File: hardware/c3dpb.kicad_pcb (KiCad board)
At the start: 4 copper layers, 100 x 75 mm, 567 parts, among them IC1 TMC5161, IC2 TMC5161, IC3 TMC5161, IC4 TMC5161, IC5 TMC5161, J1 Conn_01x01, J10 Conn_01x01, J100 Conn_01x01, J101 Conn_01x01, J102 Conn_01x01, J104 Conn_01x01, J11 Conn_01x01, J12 Conn_01x01, J13 Conn_01x01, J14 Conn_01x01, J15 Conn_01x01, J16 Conn_01x01, J17 Conn_01x01, J18 Conn_01x01, J19 Conn_01x01, J2 Conn_01x01, J20 Conn_01x01, J21 Conn_01x01, J22 Conn_01x01, J23 Conn_01x01, J24 Conn_01x01, J25 Conn_01x01, J26 Conn_01x01, J27 Conn_01x01, J28 Conn_01x01, J29 Conn_01x01, J3 Conn_01x01, J30 Conn_01x01, J31 Conn_01x01, J32 Conn_01x01, J33 Conn_01x01, J34 Conn_01x01, J35 Conn_01x01, J36 Conn_01x01, J37 Conn_01x01, J38 Conn_01x01, J39 Screw_Terminal_01x02, J4 Conn_01x01, J44 Conn_01x01, J45 Conn_01x01, J46 Conn_01x03, J47 Conn_01x03, J48 Conn_01x01, J49 Conn_01x01, J5 Conn_01x01, J50 Conn_01x01, J51 Conn_01x01, J52 Conn_01x01, J53 Conn_01x01, J54 Conn_01x01, J55 Conn_01x01, J56 Conn_01x01, J57 Conn_01x01, J58 Conn_01x01, J59 Conn_01x01, J6 Conn_01x01, J60 USB_C_Receptacle, J61 Micro_SD_Card_Det, J62 Conn_01x02, J63 Conn_01x02, J66 Conn_01x03, J67 Conn_01x03, J68 Conn_01x01, J69 Conn_01x01, J7 Conn_01x01, J70 Conn_01x01, J71 Conn_01x02, J72 Conn_01x02, J73 Conn_01x02, J74 Conn_01x02, J75 Conn_01x01, J76 Conn_01x01, J77 Conn_01x01, J78 Conn_01x01, J79 Conn_01x03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

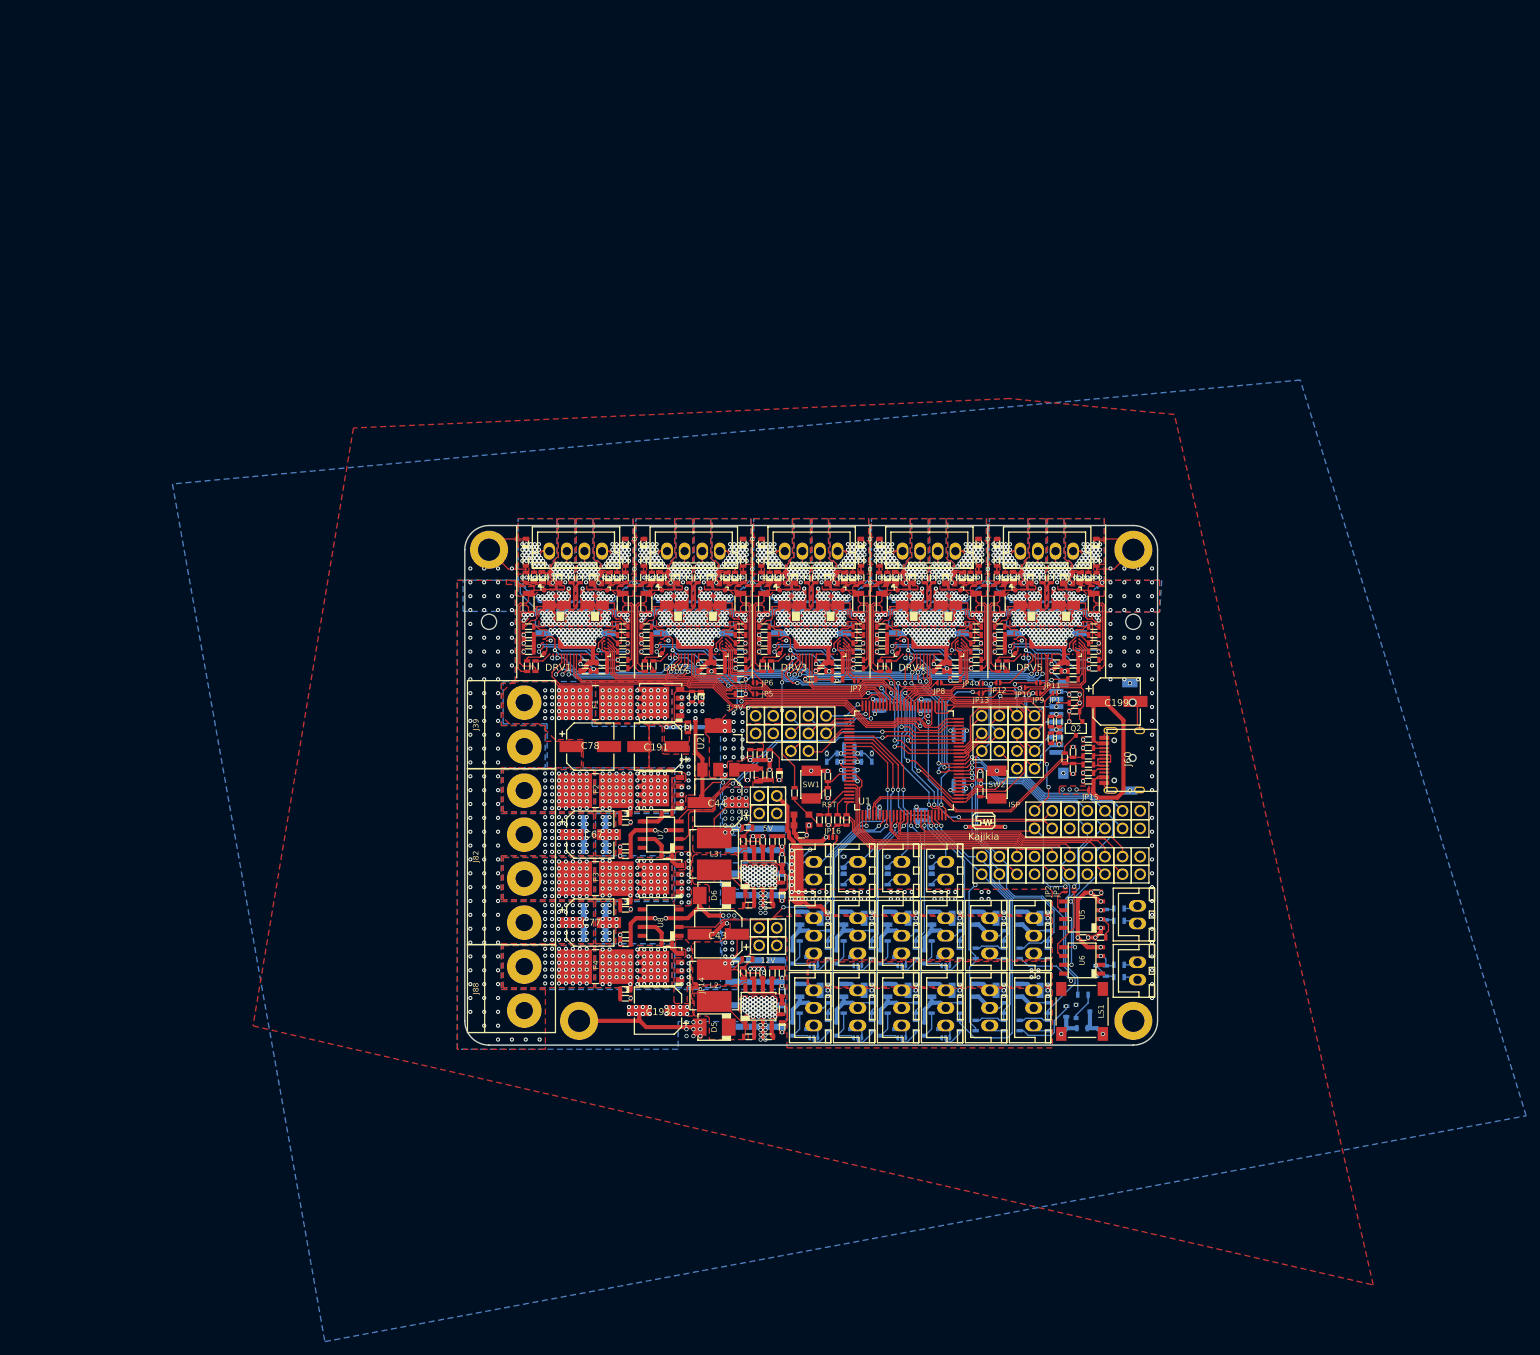
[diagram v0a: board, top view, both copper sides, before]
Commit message: layout
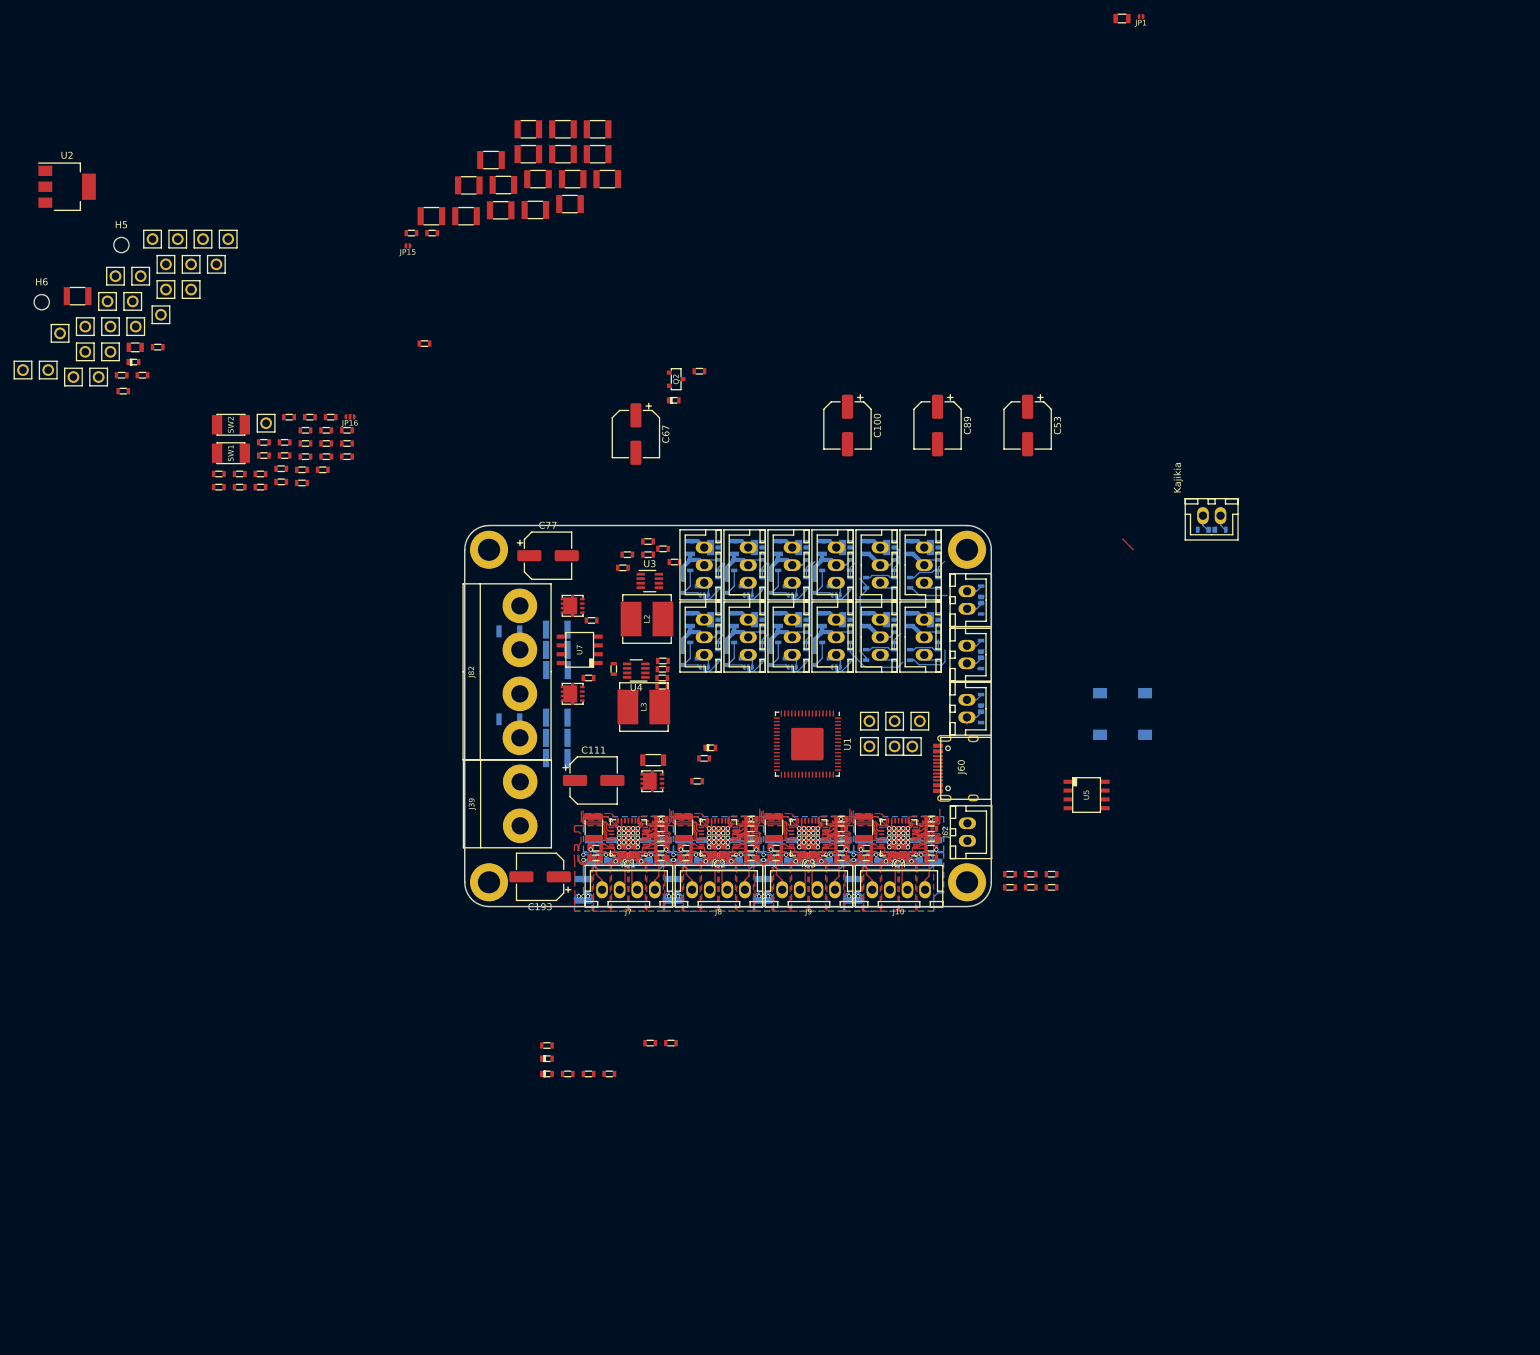
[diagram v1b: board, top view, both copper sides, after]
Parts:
- removed C130, C145, C148, C150, C151, C166, C169, C171, C172: 100n, _Generic:0603_CAP
- removed C131, C132, C134, C135, C142, C143, C147, C152, C153, C155, C156, C163, C164, C168, C173, C174, C176, C177, C184, C185: 470n, _Generic:0603_CAP
- removed C133, C136, C137, C154, C157, C158, C175, C178, C179, C186, C187, C188, C189, C190, C194, C195, C196, C197: 4.7u, _Generic:1210_CAP
- removed C138, C139, C140, C141, C159, C160, C161, C162, C180, C181, C182, C183: 470p, _Generic:0603_CAP
- removed C144, C146, C165, C167: 10u, _Generic:0603_CAP
- removed C149, C170: 22n, _Generic:0603_CAP
- removed C191, C199: 220u, Capacitor_SMD:CP_Elec_6.3x7.7
- removed D25: LED, _Generic:0603_LED
- removed D26, D27, D28, D29, D30, D31, D32, D33, D34, D35, D36, D37, D38, D39, D40, D41, D42, D43, D44, D45, D46, D47, D48, D49, D50, D51, D52, D53, D54, D55, D56, D57, D58, D59, D60, D61, D62, D63, D64, D65, D66: MSK4010, _Generic:SOD-523_DIODE
- removed D3: 3.6v, _Generic:SOD-523_DIODE
- removed D5, D6: SK54, _Generic:SMB_DIODE
- removed F4: Fuse, _Generic:SMD_Fuseholder
- removed IC5: TMC5161, footprints:QFN42L
- removed J104, J11, J12, J13, J14, J15, J16, J17, J18, J19, J20, J21, J22, J23, J25, J26, J27, J28, J29, J30, J31, J32, J33, J34, J35, J36, J37, J38, J52, J75, J76, J77, J78: Conn_01x01, _Generic:PinHeader_2.54mm_1P
- removed J61: Micro_SD_Card_Det, _Generic:HYC77-TF09-200
- removed J63: Conn_01x02, _Generic:JST_XH_2P
- removed J88: Screw_Terminal_01x02, _Generic:KF635-2P
- removed J89, J90, J91, J92, J93: Conn_01x04, _Generic:JST_XH_4P
- removed JP10, JP11, JP12, JP13, JP14, JP2, JP3, JP38, JP39, JP4, JP40, JP41, JP42, JP5, JP6, JP7, JP8, JP9: SolderJumper_2_Open, _Generic:Solder Jumper 2P
- removed L6, L7: 470, _Generic:0603_IND
- removed Q11: AON6144, _Generic:DFN5x6-8
- removed Q14: AO3400, _Generic:SOT-23
- removed R100, R109, R118, R82, R91: 2.2R, _Generic:0603_RES
- removed R101, R110, R119, R76, R77, R80, R83, R92: 1k, _Generic:0603_RES
- removed R102, R103, R104, R105, R111, R112, R113, R114, R120, R121, R122, R123, R84, R85, R86, R87, R93, R94, R95, R96: 47R, _Generic:0603_RES
- removed R106, R107, R115, R116, R124, R125, R88, R89, R97, R98: 100m, _Generic:1206_RES
- removed R108, R117, R34, R78, R81, R90, R99: 0R, _Generic:0603_RES
- removed R30, R31, R79: 10k, _Generic:0603_RES
- removed R75: 10R, _Generic:0603_RES
- removed U6: MAX6675, _Generic:SO-8
- removed U8: IR4427S, _Generic:SO-8
- removed X1: 12MHz, Oscillator:Oscillator_SMD_EuroQuartz_XO32-4Pin_3.2x2.5mm
- added FB1: Ferrite_Bead_Small, _Generic:0805_IND, F.Cu at (194.9, -23.2)
- C10, C11, C12, C13, C14, C15, C16, C17, C19, C2, C23, C24, C25, C26, C27, C31, C4, C48, C6, C7, C8, C9, L4, L5, R4, R5, R6, R7: moved to F.Cu
- C100, C111, C89: value 470n -> 100u; footprint _Generic:0603_CAP -> Capacitor_SMD:CP_Elec_6.3x7.7
- C101, C114, C90, C92: value 470n -> 470p; moved to B.Cu
- C102, C104: value 10u -> 470p
- C103: value 100n -> 470p; moved to B.Cu
- C105: value 470n -> 100n
- C106, C127, C129, C47, C52, C88: value 100n -> 4.7u; footprint _Generic:0603_CAP -> _Generic:1210_CAP; moved to B.Cu
- C107: value 22n -> 2.2u
- C109, C87: value 100n -> 22n
- C110, C121, C84: value 470n -> 4.7u; footprint _Generic:0603_CAP -> _Generic:1210_CAP; moved to B.Cu
- C112: value 4.7u -> 470p; footprint _Generic:1210_CAP -> _Generic:0603_CAP
- C113, C93: value 470n -> 470p
- C115, C91: value 4.7u -> 470p; footprint _Generic:1210_CAP -> _Generic:0603_CAP; moved to F.Cu
- C116, C94: value 4.7u -> 100n; footprint _Generic:1210_CAP -> _Generic:0603_CAP; moved to F.Cu
- C117, C118, C119, C97: value 470p -> 100n
- C120: value 470p -> 4.7u; footprint _Generic:0603_CAP -> _Generic:1210_CAP
- C122, C126: value 470n -> 4.7u; footprint _Generic:0603_CAP -> _Generic:1210_CAP
- C123, C125: value 10u -> 4.7u; footprint _Generic:0603_CAP -> _Generic:1210_CAP; moved to B.Cu
- C124, C5: value 100n -> 4.7u; footprint _Generic:0603_CAP -> _Generic:1210_CAP
- C128: value 22n -> 4.7u; footprint _Generic:0603_CAP -> _Generic:1210_CAP; moved to B.Cu
- C28: value 4.7u -> 10n; footprint _Generic:1210_CAP -> _Generic:0603_CAP; moved to F.Cu
- C29: value 100n -> 47p
- C3: value 220p -> 4.7u; footprint _Generic:0603_CAP -> _Generic:1210_CAP
- C30, C38: value 100n -> 22u; footprint _Generic:0603_CAP -> _Generic:1210_CAP
- C32, C41, C42: value 4.7u -> 22u; moved to F.Cu
- C33, C34: value 22n -> 22u; footprint _Generic:0603_CAP -> _Generic:1210_CAP
- C35, C36: value 12p -> 22u; footprint _Generic:0603_CAP -> _Generic:1210_CAP
- C37: value 100n -> 10n
- C39: value DNP -> 47p
- C40: value DNP -> 22u; footprint _Generic:0603_CAP -> _Generic:1210_CAP
- C43, C44: value 220u -> 22u; footprint Capacitor_SMD:CP_Elec_6.3x7.7 -> _Generic:1210_CAP
- C46, C83: value 10u -> 100n
- C49: value 10u -> 2.2u
- C50: value 12p -> 100n
- C51: value 12p -> 22n
- C53: value 22n -> 100u; footprint _Generic:0603_CAP -> Capacitor_SMD:CP_Elec_6.3x7.7; moved to F.Cu
- C78: value 220u -> 470p; footprint Capacitor_SMD:CP_Elec_6.3x7.7 -> _Generic:0603_CAP; moved to B.Cu
- C80: value 100p -> 470p
- C81: value 10u -> 470p; moved to B.Cu
- C82: value 100n -> 470p
- C85: value 100n -> 2.2u
- C86: value 22n -> 100n
- C96: value 470p -> 2.2u
- C98: value 470p -> 22n
- C99: value 470p -> 4.7u; footprint _Generic:0603_CAP -> _Generic:1210_CAP; moved to B.Cu
- D2: value 3.6v -> MSK4010
- F1: footprint _Generic:SMD_Fuseholder -> _Generic:1206_RES
- F2, F3: footprint _Generic:SMD_Fuseholder -> _Generic:1206_RES; moved to B.Cu
- IC1, IC2, IC3, IC4: value TMC5161 -> TMC2209; footprint footprints:QFN42L -> Package_DFN_QFN:QFN-28-1EP_5x5mm_P0.5mm_EP3.35x3.35mm
- J10, J7, J8, J9: value Conn_01x01 -> Conn_01x04; footprint _Generic:PinHeader_2.54mm_1P -> _Generic:JST_XH_4P
- LS1: moved to B.Cu
- Q1, Q6, Q7: value AON6144 -> AON7418; footprint _Generic:DFN5x6-8 -> _Generic:DFN3x3A_8L_EP1_P
- Q2: value AO3401 -> AO3400
- R10: value 47k -> 1k
- R11: value 47k -> 100k
- R12, R17: value 140k -> 100k
- R13: value 140k -> 13.3k
- R16: value 100k -> 1k
- R18: value 10k -> 4.7k
- R19: value 52.3k -> 120m; footprint _Generic:0603_RES -> _Generic:1206_RES; moved to B.Cu
- R20, R27, R29: value 10k -> 120m; footprint _Generic:0603_RES -> _Generic:1206_RES; moved to B.Cu
- R24, R25: value 47R -> 120m; footprint _Generic:0603_RES -> _Generic:1206_RES; moved to B.Cu
- R26: value 1.5k -> 120m; footprint _Generic:0603_RES -> _Generic:1206_RES; moved to B.Cu
- R28: value 47k -> 120m; footprint _Generic:0603_RES -> _Generic:1206_RES; moved to B.Cu
- R8: value 10k -> 100k
- R9: value 100k -> 1meg
- U1: value LPC1769FBD100 -> ATSAMD51J19A-M; footprint Package_QFP:LQFP-100_14x14mm_P0.5mm -> Package_DFN_QFN:QFN-64-1EP_9x9mm_P0.5mm_EP4.7x4.7mm
- U3, U4: value AOZ1284 -> SY8303; footprint _Generic:SO-8-EP1 -> Package_TO_SOT_SMD:TSOT-23-8
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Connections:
- net Net-(IC2-Pad9) renamed /Driver 3/AD0
- net Net-(IC4-Pad9) renamed /Driver 1/AD0
- C101 pad 1: +24V -> Net-(C101-Pad1)
- C103 pad 1: Net-(C102-Pad1) -> Net-(C103-Pad1)
- C104 pad 1: /Stepper Driver/Driver2/5V_out -> Net-(C104-Pad1)
- C105 pad 1: /Stepper Driver/Driver2/VCC -> GND
- C105 pad 2: GND -> +24V
- C106 pad 1: +3V3 -> +24V
- C107 pad 2: Net-(C107-Pad2) -> GND
- C109 pad 1: GND -> Net-(C109-Pad1)
- C109 pad 2: +24V -> Net-(C109-Pad2)
- C110 pad 1: /Stepper Driver/Driver2/OA2 -> +24V
- C110 pad 2: Net-(C110-Pad2) -> GND
- C111 pad 1: /Stepper Driver/Driver2/OB2 -> +24V
- C111 pad 2: Net-(C111-Pad2) -> GND
- C112 pad 1: +24V -> Net-(C112-Pad1)
- C113 pad 1: /Stepper Driver/Driver2/OA1 -> Net-(C113-Pad1)
- C113 pad 2: Net-(C113-Pad2) -> GND
- C114 pad 1: /Stepper Driver/Driver2/OB1 -> Net-(C114-Pad1)
- C114 pad 2: Net-(C114-Pad2) -> GND
- C115 pad 1: +24V -> Net-(C115-Pad1)
- C116 pad 1: +24V -> GND
- C116 pad 2: GND -> +24V
- C117 pad 1: /Stepper Driver/Driver2/OA2 -> GND
- C117 pad 2: GND -> +24V
- C118 pad 1: /Stepper Driver/Driver2/OB2 -> GND
- C118 pad 2: GND -> +24V
- C119 pad 1: /Stepper Driver/Driver2/OA1 -> GND
- C119 pad 2: GND -> +24V
- C120 pad 1: /Stepper Driver/Driver2/OB1 -> +24V
- C123 pad 1: Net-(C123-Pad1) -> +24V
- C124 pad 1: Net-(C123-Pad1) -> +24V
- C125 pad 1: /Stepper Driver/Driver3/5V_out -> +24V
- C126 pad 1: /Stepper Driver/Driver3/VCC -> +24V
- C127 pad 1: +3V3 -> +24V
- C128 pad 2: Net-(C128-Pad2) -> DCIN-
- C129 pad 2: +24V -> DCIN-
- C192 pad 1: +24V -> Net-(C129-Pad1)
- C198 pad 1: VBUS -> Net-(C198-Pad1)
- C28 pad 1: +24V -> Net-(C28-Pad1)
- C28 pad 2: GND -> Net-(C28-Pad2)
- C29 pad 1: Net-(C29-Pad1) -> +5V
- C29 pad 2: GND -> Net-(C29-Pad2)
- C3 pad 1: /LPC_CLK -> +24V
- C30 pad 1: Net-(C30-Pad1) -> +12V
- C30 pad 2: GND -> Net-(C30-Pad2)
- C32 pad 1: +24V -> +12V
- C33 pad 1: Net-(C33-Pad1) -> +5V
- C33 pad 2: GND -> Net-(C33-Pad2)
- C34 pad 1: Net-(C34-Pad1) -> +5V
- C35 pad 1: Net-(C35-Pad1) -> +12V
- C35 pad 2: Net-(C35-Pad2) -> Net-(C30-Pad2)
- C36 pad 1: Net-(C36-Pad1) -> +12V
- C36 pad 2: Net-(C36-Pad2) -> GND
- C38 pad 1: Net-(C38-Pad1) -> +5V
- C38 pad 2: Net-(C38-Pad2) -> Net-(C33-Pad2)
- C40 pad 2: Net-(C40-Pad2) -> GND
- C41 pad 2: GND -> Net-(C30-Pad2)
- C42 pad 1: +5V -> +12V
- C43 pad 1: +12V -> +5V
- C43 pad 2: GND -> Net-(C33-Pad2)
- C46 pad 1: VBUS -> GND
- C46 pad 2: GND -> +24V
- C47 pad 1: +3V3 -> +24V
- C49 pad 1: +3V3 -> Net-(C49-Pad1)
- C5 pad 1: +3V3 -> +24V
- C50 pad 1: /USB_D+ -> Net-(C50-Pad1)
- C50 pad 2: GND -> +24V
- C51 pad 1: /USB_D- -> Net-(C51-Pad1)
- C51 pad 2: GND -> Net-(C51-Pad2)
- C52 pad 1: +3V3 -> +24V
- C53 pad 1: Net-(C53-Pad1) -> +24V
- C53 pad 2: Net-(C53-Pad2) -> GND
- C68 pad 1: +24V -> Net-(C129-Pad1)
- C69 pad 1: +24V -> Net-(C128-Pad1)
- C78 pad 1: +24V -> Net-(C78-Pad1)
- C78 pad 2: DCIN- -> GND
- C79 pad 1: +24V -> Net-(C128-Pad1)
- C80 pad 1: /LPC_CLK -> Net-(C80-Pad1)
- C80 pad 2: Net-(C80-Pad2) -> GND
- C82 pad 1: Net-(C81-Pad1) -> Net-(C82-Pad1)
- C83 pad 1: /Stepper Driver/Driver1/5V_out -> GND
- C83 pad 2: GND -> +24V
- C84 pad 1: /Stepper Driver/Driver1/VCC -> +24V
- C85 pad 1: +3V3 -> Net-(C85-Pad1)
- C86 pad 2: Net-(C86-Pad2) -> +24V
- C87 pad 2: +24V -> Net-(C87-Pad2)
- C88 pad 1: GND -> +24V
- C88 pad 2: +24V -> GND
- C89 pad 1: /Stepper Driver/Driver1/OA2 -> +24V
- C89 pad 2: Net-(C89-Pad2) -> GND
- C90 pad 1: /Stepper Driver/Driver1/OB2 -> Net-(C90-Pad1)
- C90 pad 2: Net-(C90-Pad2) -> GND
- C91 pad 1: +24V -> Net-(C91-Pad1)
- C92 pad 1: /Stepper Driver/Driver1/OA1 -> Net-(C92-Pad1)
- C92 pad 2: Net-(C92-Pad2) -> GND
- C93 pad 1: /Stepper Driver/Driver1/OB1 -> Net-(C93-Pad1)
- C93 pad 2: Net-(C93-Pad2) -> GND
- C94 pad 1: +24V -> GND
- C94 pad 2: GND -> +24V
- C96 pad 1: /Stepper Driver/Driver1/OA2 -> Net-(C96-Pad1)
- C97 pad 1: /Stepper Driver/Driver1/OB2 -> Net-(C97-Pad1)
- C97 pad 2: GND -> +24V
- C98 pad 1: /Stepper Driver/Driver1/OA1 -> Net-(C98-Pad1)
- C98 pad 2: GND -> Net-(C98-Pad2)
- C99 pad 1: /Stepper Driver/Driver1/OB1 -> +24V
- D2 pad 1: Net-(C29-Pad1) -> +3V3
- D2 pad 2: GND -> Net-(D2-Pad2)
- F2 pad 1: Net-(F2-Pad1) -> Net-(C128-Pad1)
- F2 pad 2: Net-(D18-Pad1) -> +24V
- F3 pad 1: Net-(F3-Pad1) -> Net-(C129-Pad1)
- F3 pad 2: Net-(D19-Pad1) -> +24V
- IC1 pad 1: Net-(C93-Pad2) -> Net-(C82-Pad1)
- IC1 pad 10: Net-(IC1-Pad10) -> /Driver 2/AD1
- IC1 pad 11: /Stepper Driver/Driver1/SRBH -> /DRV2_DIAG
- IC1 pad 14: /DRV_CLK -> /DRV_UART
- IC1 pad 15: /DRV1_CS -> Net-(IC1-Pad15)
- IC1 pad 16: /DRV_SCK -> /DRV2_STEP
- IC1 pad 17: /DRV_MOSI -> Net-(IC1-Pad17)
- IC1 pad 18: /DRV_MISO -> GND
- IC1 pad 19: /DRV1_STEP -> /DRV2_DIR
- IC1 pad 2: Net-(C81-Pad1) -> /DRV2_EN
- IC1 pad 20: /DRV1_DIR -> Net-(IC1-Pad20)
- IC1 pad 21: +3V3 -> Net-(C80-Pad1)
- IC1 pad 22: +3V3 -> +24V
- IC1 pad 23: +3V3 -> Net-(IC1-Pad23)
- IC1 pad 24: GND -> Net-(C78-Pad1)
- IC1 pad 25: GND -> Net-(IC1-Pad25)
- IC1 pad 26: GND -> Net-(C81-Pad1)
- IC1 pad 28: Net-(IC1-Pad28) -> +24V
- IC1 pad 29: /Stepper Driver/DRV1_DIAG1 -> GND
- IC1 pad 3: Net-(IC1-Pad3) -> GND
- IC1 pad 4: Net-(C81-Pad1) -> Net-(C51-Pad2)
- IC1 pad 5: /Stepper Driver/Driver1/5V_out -> Net-(C51-Pad1)
- IC1 pad 6: /Stepper Driver/Driver1/5V_out -> Net-(C50-Pad1)
- IC1 pad 7: GND -> Net-(IC1-Pad7)
- IC1 pad 8: Net-(IC1-Pad8) -> Net-(C49-Pad1)
- IC1 pad 9: Net-(IC1-Pad9) -> +3V3
- IC2 pad 1: Net-(C114-Pad2) -> Net-(C93-Pad1)
- IC2 pad 10: Net-(IC2-Pad10) -> +3V3
- IC2 pad 11: /Stepper Driver/Driver2/SRBH -> /DRV3_DIAG
- IC2 pad 14: /DRV_CLK -> /DRV_UART
- IC2 pad 15: /DRV2_CS -> Net-(IC2-Pad15)
- IC2 pad 16: /DRV_SCK -> /DRV3_STEP
- IC2 pad 17: /DRV_MOSI -> Net-(IC2-Pad17)
- IC2 pad 18: /DRV_MISO -> GND
- IC2 pad 19: /DRV2_STEP -> /DRV3_DIR
- IC2 pad 2: Net-(C102-Pad1) -> /DRV3_EN
- IC2 pad 20: /DRV2_DIR -> Net-(IC2-Pad20)
- IC2 pad 21: +3V3 -> Net-(C91-Pad1)
- IC2 pad 22: +3V3 -> +24V
- IC2 pad 23: +3V3 -> Net-(IC2-Pad23)
- IC2 pad 24: GND -> Net-(C90-Pad1)
- IC2 pad 25: GND -> Net-(IC2-Pad25)
- IC2 pad 26: GND -> Net-(C92-Pad1)
- IC2 pad 28: Net-(IC2-Pad28) -> +24V
- IC2 pad 29: /Stepper Driver/DRV2_DIAG1 -> GND
- IC2 pad 3: Net-(IC2-Pad3) -> GND
- IC2 pad 4: Net-(C102-Pad1) -> Net-(C87-Pad2)
- IC2 pad 5: /Stepper Driver/Driver2/5V_out -> Net-(C87-Pad1)
- IC2 pad 6: /Stepper Driver/Driver2/5V_out -> Net-(C86-Pad1)
- IC2 pad 7: GND -> Net-(IC2-Pad7)
- IC2 pad 8: Net-(IC2-Pad8) -> Net-(C85-Pad1)
- IC3 pad 1: Net-(C135-Pad2) -> Net-(C104-Pad1)
- IC3 pad 10: Net-(IC3-Pad10) -> +3V3
- IC3 pad 11: /Stepper Driver/Driver3/SRBH -> /DRV4_DIAG
- IC3 pad 14: /DRV_CLK -> /DRV_UART
- IC3 pad 15: /DRV3_CS -> Net-(IC3-Pad15)
- IC3 pad 16: /DRV_SCK -> /DRV4_STEP
- IC3 pad 17: /DRV_MOSI -> Net-(IC3-Pad17)
- IC3 pad 18: /DRV_MISO -> GND
- IC3 pad 19: /DRV3_STEP -> /DRV4_DIR
- IC3 pad 2: Net-(C123-Pad1) -> /DRV4_EN
- IC3 pad 20: /DRV3_DIR -> Net-(IC3-Pad20)
- IC3 pad 21: +3V3 -> Net-(C102-Pad1)
- IC3 pad 22: +3V3 -> +24V
- IC3 pad 23: +3V3 -> Net-(IC3-Pad23)
- IC3 pad 24: GND -> Net-(C101-Pad1)
- IC3 pad 25: GND -> Net-(IC3-Pad25)
- IC3 pad 26: GND -> Net-(C103-Pad1)
- IC3 pad 28: Net-(IC3-Pad28) -> +24V
- IC3 pad 29: /Stepper Driver/DRV3_DIAG1 -> GND
- IC3 pad 3: Net-(IC3-Pad3) -> GND
- IC3 pad 4: Net-(C123-Pad1) -> Net-(C98-Pad2)
- IC3 pad 5: /Stepper Driver/Driver3/5V_out -> Net-(C98-Pad1)
- IC3 pad 6: /Stepper Driver/Driver3/5V_out -> Net-(C97-Pad1)
- IC3 pad 7: GND -> Net-(IC3-Pad7)
- IC3 pad 8: Net-(IC3-Pad8) -> Net-(C96-Pad1)
- IC3 pad 9: Net-(IC3-Pad9) -> +3V3
- IC4 pad 1: Net-(C156-Pad2) -> Net-(C115-Pad1)
- IC4 pad 10: Net-(IC4-Pad10) -> /Driver 1/AD1
- IC4 pad 11: /Stepper Driver/Driver4/SRBH -> /DRV1_DIAG
- IC4 pad 14: /DRV_CLK -> /DRV_UART
- IC4 pad 15: /DRV4_CS -> Net-(IC4-Pad15)
- IC4 pad 16: /DRV_SCK -> /DRV1_STEP
- IC4 pad 17: /DRV_MOSI -> Net-(IC4-Pad17)
- IC4 pad 18: /DRV_MISO -> GND
- IC4 pad 19: /DRV4_STEP -> /DRV1_DIR
- IC4 pad 2: Net-(C144-Pad1) -> /DRV1_EN
- IC4 pad 20: /DRV4_DIR -> Net-(IC4-Pad20)
- IC4 pad 21: +3V3 -> Net-(C113-Pad1)
- IC4 pad 22: +3V3 -> +24V
- IC4 pad 23: +3V3 -> Net-(IC4-Pad23)
- IC4 pad 24: GND -> Net-(C112-Pad1)
- IC4 pad 25: GND -> Net-(IC4-Pad25)
- IC4 pad 26: GND -> Net-(C114-Pad1)
- IC4 pad 28: Net-(IC4-Pad28) -> +24V
- IC4 pad 29: /Stepper Driver/DRV4_DIAG1 -> GND
- IC4 pad 3: Net-(IC4-Pad3) -> GND
- IC4 pad 4: Net-(C144-Pad1) -> Net-(C109-Pad2)
- IC4 pad 5: /Stepper Driver/Driver4/5V_out -> Net-(C109-Pad1)
- IC4 pad 6: /Stepper Driver/Driver4/5V_out -> Net-(C108-Pad1)
- IC4 pad 7: GND -> Net-(IC4-Pad7)
- IC4 pad 8: Net-(IC4-Pad8) -> Net-(C107-Pad1)
- J1 pad 1: /P0.0_END -> /SWCLK
- J10 pad 1: /DRV5_CS -> Net-(C115-Pad1)
- J2 pad 1: /P0.1_END -> /BUZZER
- J3 pad 1: /P0.2 -> Net-(J3-Pad1)
- J4 pad 1: /P0.3 -> Net-(J4-Pad1)
- J5 pad 1: /SD_CS -> Net-(J5-Pad1)
- J6 pad 1: /SD_SCK -> Net-(J6-Pad1)
- J60 pad A4: VBUS -> Net-(C198-Pad1)
- J60 pad A6: Net-(J60-PadA6) -> /USB_D+
- J60 pad A7: Net-(J60-PadA7) -> /USB_D-
- J60 pad A9: VBUS -> Net-(C198-Pad1)
- J60 pad B4: VBUS -> Net-(C198-Pad1)
- J60 pad B6: Net-(J60-PadA6) -> /USB_D+
- J60 pad B7: Net-(J60-PadA7) -> /USB_D-
- J60 pad B9: VBUS -> Net-(C198-Pad1)
- J60 pad S1: GND -> Net-(FB1-Pad2)
- J7 pad 1: /SD_MISO -> Net-(C82-Pad1)
- J8 pad 1: /SD_MOSI -> Net-(C93-Pad1)
- J82 pad 1: Net-(F2-Pad1) -> Net-(D18-Pad1)
- J82 pad 2: +24V -> Net-(C128-Pad1)
- J82 pad 3: Net-(F3-Pad1) -> Net-(D19-Pad1)
- J82 pad 4: +24V -> Net-(C129-Pad1)
- J9 pad 1: /DRV_SCK -> Net-(C104-Pad1)
- JP1 pad 1: /Interfaces/SD_DETECT -> /BUZZER
- JP1 pad 2: /P4.29 -> Net-(JP1-Pad2)
- JP15 pad 1: VBUS -> Net-(C198-Pad1)
- L3 pad 1: Net-(C38-Pad2) -> Net-(C28-Pad2)
- LS1 pad 1: Net-(D26-Pad1) -> +3V3
- LS1 pad 2: Net-(D26-Pad2) -> Net-(D2-Pad2)
- Q2 pad 1: /USB_CON -> Net-(Q2-Pad1)
- Q2 pad 2: +3V3 -> GND
- Q2 pad 3: Net-(Q2-Pad3) -> Net-(D2-Pad2)
- R10 pad 1: Net-(R10-Pad1) -> +3V3
- R10 pad 2: GND -> /SWCLK
- R12 pad 1: +24V -> +5V
- R12 pad 2: Net-(C29-Pad1) -> Net-(C29-Pad2)
- R13 pad 1: +24V -> Net-(C29-Pad2)
- R13 pad 2: Net-(C30-Pad1) -> GND
- R15 pad 1: Net-(C35-Pad2) -> Net-(R15-Pad1)
- R16 pad 1: Net-(C36-Pad2) -> Net-(Q2-Pad1)
- R16 pad 2: GND -> Net-(JP1-Pad2)
- R19 pad 1: +5V -> Net-(IC1-Pad27)
- R19 pad 2: Net-(C40-Pad2) -> GND
- R20 pad 1: Net-(C40-Pad2) -> Net-(IC1-Pad23)
- R24 pad 1: /USB_D- -> Net-(IC2-Pad27)
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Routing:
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- added copper zone on B.Cu, net Net-(C101-Pad1)
- added copper zone on F.Cu, net Net-(C101-Pad1)
- added copper zone on F.Cu, net Net-(C102-Pad1)
- added copper zone on B.Cu, net Net-(C103-Pad1)
- added copper zone on F.Cu, net Net-(C103-Pad1)
- added copper zone on F.Cu, net Net-(C104-Pad1)
- added copper zone on F.Cu, net Net-(C107-Pad1)
- added copper zone on F.Cu, net Net-(C108-Pad1)
- added copper zone on F.Cu, net Net-(C109-Pad1)
- added copper zone on F.Cu, net Net-(C109-Pad2)
- added copper zone on B.Cu, net Net-(C112-Pad1)
- added copper zone on F.Cu, net Net-(C112-Pad1)
- added copper zone on F.Cu, net Net-(C113-Pad1)
- added copper zone on B.Cu, net Net-(C114-Pad1)
- added copper zone on F.Cu, net Net-(C114-Pad1)
- added copper zone on F.Cu, net Net-(C115-Pad1)
- added copper zone on F.Cu, net Net-(C49-Pad1)
- added copper zone on F.Cu, net Net-(C50-Pad1)
- added copper zone on F.Cu, net Net-(C51-Pad1)
- added copper zone on F.Cu, net Net-(C51-Pad2)
- added copper zone on B.Cu, net Net-(C78-Pad1)
- added copper zone on F.Cu, net Net-(C78-Pad1)
- added copper zone on F.Cu, net Net-(C80-Pad1)
- added copper zone on B.Cu, net Net-(C81-Pad1)
- added copper zone on F.Cu, net Net-(C81-Pad1)
- added copper zone on F.Cu, net Net-(C82-Pad1)
- added copper zone on F.Cu, net Net-(C85-Pad1)
- added copper zone on F.Cu, net Net-(C86-Pad1)
- added copper zone on F.Cu, net Net-(C87-Pad1)
- added copper zone on F.Cu, net Net-(C87-Pad2)
- added copper zone on B.Cu, net Net-(C90-Pad1)
- added copper zone on F.Cu, net Net-(C90-Pad1)
- added copper zone on F.Cu, net Net-(C91-Pad1)
- added copper zone on B.Cu, net Net-(C92-Pad1)
- added copper zone on F.Cu, net Net-(C92-Pad1)
- added copper zone on F.Cu, net Net-(C93-Pad1)
- added copper zone on F.Cu, net Net-(C96-Pad1)
- added copper zone on F.Cu, net Net-(C97-Pad1)
- added copper zone on F.Cu, net Net-(C98-Pad1)
- added copper zone on F.Cu, net Net-(C98-Pad2)
- added copper zone on B.Cu, net Net-(IC1-Pad23)
- added copper zone on F.Cu, net Net-(IC1-Pad23)
- added copper zone on B.Cu, net Net-(IC1-Pad27)
- added copper zone on F.Cu, net Net-(IC1-Pad27)
- added copper zone on B.Cu, net Net-(IC2-Pad23)
- added copper zone on F.Cu, net Net-(IC2-Pad23)
- added copper zone on B.Cu, net Net-(IC2-Pad27)
- added copper zone on F.Cu, net Net-(IC2-Pad27)
- added copper zone on B.Cu, net Net-(IC3-Pad23)
- added copper zone on F.Cu, net Net-(IC3-Pad23)
- added copper zone on B.Cu, net Net-(IC3-Pad27)
- added copper zone on F.Cu, net Net-(IC3-Pad27)
- added copper zone on B.Cu, net Net-(IC4-Pad23)
- added copper zone on F.Cu, net Net-(IC4-Pad23)
- added copper zone on B.Cu, net Net-(IC4-Pad27)
- added copper zone on F.Cu, net Net-(IC4-Pad27)
- removed copper zone on B.Cu, net +12V
- removed copper zone on F.Cu, net +12V
- removed copper zone on In2.Cu, net +12V
- removed copper zone on In1.Cu, net +24V
- removed copper zone on In2.Cu, net +24V
- removed copper zone on F.Cu, net +3V3
- removed copper zone on In2.Cu, net +3V3
- removed copper zone on B.Cu, net +5V
- removed copper zone on F.Cu, net +5V
- removed copper zone on In2.Cu, net +5V
- removed copper zone on B.Cu, net /Stepper Driver/Driver1/OA1
- removed copper zone on F.Cu, net /Stepper Driver/Driver1/OA1
- removed copper zone on In1.Cu, net /Stepper Driver/Driver1/OA1
- removed copper zone on In2.Cu, net /Stepper Driver/Driver1/OA1
- removed copper zone on B.Cu, net /Stepper Driver/Driver1/OA2
- removed copper zone on F.Cu, net /Stepper Driver/Driver1/OA2
- removed copper zone on In1.Cu, net /Stepper Driver/Driver1/OA2
- removed copper zone on In2.Cu, net /Stepper Driver/Driver1/OA2
- removed copper zone on B.Cu, net /Stepper Driver/Driver1/OB1
- removed copper zone on F.Cu, net /Stepper Driver/Driver1/OB1
- removed copper zone on In1.Cu, net /Stepper Driver/Driver1/OB1
- removed copper zone on In2.Cu, net /Stepper Driver/Driver1/OB1
- removed copper zone on B.Cu, net /Stepper Driver/Driver1/OB2
- removed copper zone on F.Cu, net /Stepper Driver/Driver1/OB2
- removed copper zone on In1.Cu, net /Stepper Driver/Driver1/OB2
- removed copper zone on In2.Cu, net /Stepper Driver/Driver1/OB2
- removed copper zone on F.Cu, net /Stepper Driver/Driver1/RSA
- removed copper zone on F.Cu, net /Stepper Driver/Driver1/RSB
- removed copper zone on B.Cu, net /Stepper Driver/Driver2/OA1
- removed copper zone on F.Cu, net /Stepper Driver/Driver2/OA1
- removed copper zone on In1.Cu, net /Stepper Driver/Driver2/OA1
- removed copper zone on In2.Cu, net /Stepper Driver/Driver2/OA1
- removed copper zone on B.Cu, net /Stepper Driver/Driver2/OA2
- removed copper zone on F.Cu, net /Stepper Driver/Driver2/OA2
- removed copper zone on In1.Cu, net /Stepper Driver/Driver2/OA2
- removed copper zone on In2.Cu, net /Stepper Driver/Driver2/OA2
- removed copper zone on B.Cu, net /Stepper Driver/Driver2/OB1
- removed copper zone on F.Cu, net /Stepper Driver/Driver2/OB1
- removed copper zone on In1.Cu, net /Stepper Driver/Driver2/OB1
- removed copper zone on In2.Cu, net /Stepper Driver/Driver2/OB1
- removed copper zone on B.Cu, net /Stepper Driver/Driver2/OB2
- removed copper zone on F.Cu, net /Stepper Driver/Driver2/OB2
- removed copper zone on In1.Cu, net /Stepper Driver/Driver2/OB2
- removed copper zone on In2.Cu, net /Stepper Driver/Driver2/OB2
- removed copper zone on F.Cu, net /Stepper Driver/Driver2/RSA
- removed copper zone on F.Cu, net /Stepper Driver/Driver2/RSB
- removed copper zone on B.Cu, net /Stepper Driver/Driver3/OA1
- removed copper zone on F.Cu, net /Stepper Driver/Driver3/OA1
- removed copper zone on In1.Cu, net /Stepper Driver/Driver3/OA1
- removed copper zone on In2.Cu, net /Stepper Driver/Driver3/OA1
- removed copper zone on B.Cu, net /Stepper Driver/Driver3/OA2
- removed copper zone on F.Cu, net /Stepper Driver/Driver3/OA2
- removed copper zone on In1.Cu, net /Stepper Driver/Driver3/OA2
- removed copper zone on In2.Cu, net /Stepper Driver/Driver3/OA2
- removed copper zone on B.Cu, net /Stepper Driver/Driver3/OB1
- removed copper zone on F.Cu, net /Stepper Driver/Driver3/OB1
- removed copper zone on In1.Cu, net /Stepper Driver/Driver3/OB1
- removed copper zone on In2.Cu, net /Stepper Driver/Driver3/OB1
- removed copper zone on B.Cu, net /Stepper Driver/Driver3/OB2
- removed copper zone on F.Cu, net /Stepper Driver/Driver3/OB2
- removed copper zone on In1.Cu, net /Stepper Driver/Driver3/OB2
- removed copper zone on In2.Cu, net /Stepper Driver/Driver3/OB2
- removed copper zone on F.Cu, net /Stepper Driver/Driver3/RSA
- removed copper zone on F.Cu, net /Stepper Driver/Driver3/RSB
- removed copper zone on B.Cu, net /Stepper Driver/Driver4/OA1
- removed copper zone on F.Cu, net /Stepper Driver/Driver4/OA1
- removed copper zone on In1.Cu, net /Stepper Driver/Driver4/OA1
- removed copper zone on In2.Cu, net /Stepper Driver/Driver4/OA1
- removed copper zone on B.Cu, net /Stepper Driver/Driver4/OA2
- removed copper zone on F.Cu, net /Stepper Driver/Driver4/OA2
- removed copper zone on In1.Cu, net /Stepper Driver/Driver4/OA2
- removed copper zone on In2.Cu, net /Stepper Driver/Driver4/OA2
- removed copper zone on B.Cu, net /Stepper Driver/Driver4/OB1
- removed copper zone on F.Cu, net /Stepper Driver/Driver4/OB1
- removed copper zone on In1.Cu, net /Stepper Driver/Driver4/OB1
- removed copper zone on In2.Cu, net /Stepper Driver/Driver4/OB1
- removed copper zone on B.Cu, net /Stepper Driver/Driver4/OB2
- removed copper zone on F.Cu, net /Stepper Driver/Driver4/OB2
- removed copper zone on In1.Cu, net /Stepper Driver/Driver4/OB2
- removed copper zone on In2.Cu, net /Stepper Driver/Driver4/OB2
- removed copper zone on F.Cu, net /Stepper Driver/Driver4/RSA
- removed copper zone on F.Cu, net /Stepper Driver/Driver4/RSB
- removed copper zone on B.Cu, net /Stepper Driver/Driver5/OA1
- removed copper zone on F.Cu, net /Stepper Driver/Driver5/OA1
- removed copper zone on In1.Cu, net /Stepper Driver/Driver5/OA1
- removed copper zone on In2.Cu, net /Stepper Driver/Driver5/OA1
- removed copper zone on B.Cu, net /Stepper Driver/Driver5/OA2
- removed copper zone on F.Cu, net /Stepper Driver/Driver5/OA2
- removed copper zone on In1.Cu, net /Stepper Driver/Driver5/OA2
- removed copper zone on In2.Cu, net /Stepper Driver/Driver5/OA2
- removed copper zone on B.Cu, net /Stepper Driver/Driver5/OB1
- removed copper zone on F.Cu, net /Stepper Driver/Driver5/OB1
- removed copper zone on In1.Cu, net /Stepper Driver/Driver5/OB1
- removed copper zone on In2.Cu, net /Stepper Driver/Driver5/OB1
- removed copper zone on B.Cu, net /Stepper Driver/Driver5/OB2
- removed copper zone on F.Cu, net /Stepper Driver/Driver5/OB2
- removed copper zone on In1.Cu, net /Stepper Driver/Driver5/OB2
- removed copper zone on In2.Cu, net /Stepper Driver/Driver5/OB2
- removed copper zone on F.Cu, net /Stepper Driver/Driver5/RSA
- removed copper zone on F.Cu, net /Stepper Driver/Driver5/RSB
- removed copper zone on B.Cu, net DCIN-
- removed copper zone on F.Cu, net DCIN-
- removed copper zone on In1.Cu, net DCIN-
- removed copper zone on In2.Cu, net DCIN-
- removed copper zone on In1.Cu, net GND
- removed copper zone on In2.Cu, net GND
- removed copper zone on F.Cu, net Net-(C37-Pad2)
- removed copper zone on F.Cu, net Net-(C38-Pad2)
- removed copper zone on B.Cu, net Net-(D18-Pad1)
- removed copper zone on F.Cu, net Net-(D18-Pad1)
- removed copper zone on In1.Cu, net Net-(D18-Pad1)
- removed copper zone on In2.Cu, net Net-(D18-Pad1)
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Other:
- board size 100 x 75 mm -> 76 x 55 mm
- net class 24v removed
- board text removed: "3.3V"
- board text removed: "DRV1"
- board text removed: "DRV2"
- board text removed: "DRV3"
- board text removed: "DRV4"
- board text removed: "DRV5"
- board text removed: "ISP"
- board text removed: "RST"
- board text removed: "TH1"
- board text removed: "TH2"

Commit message: power reg
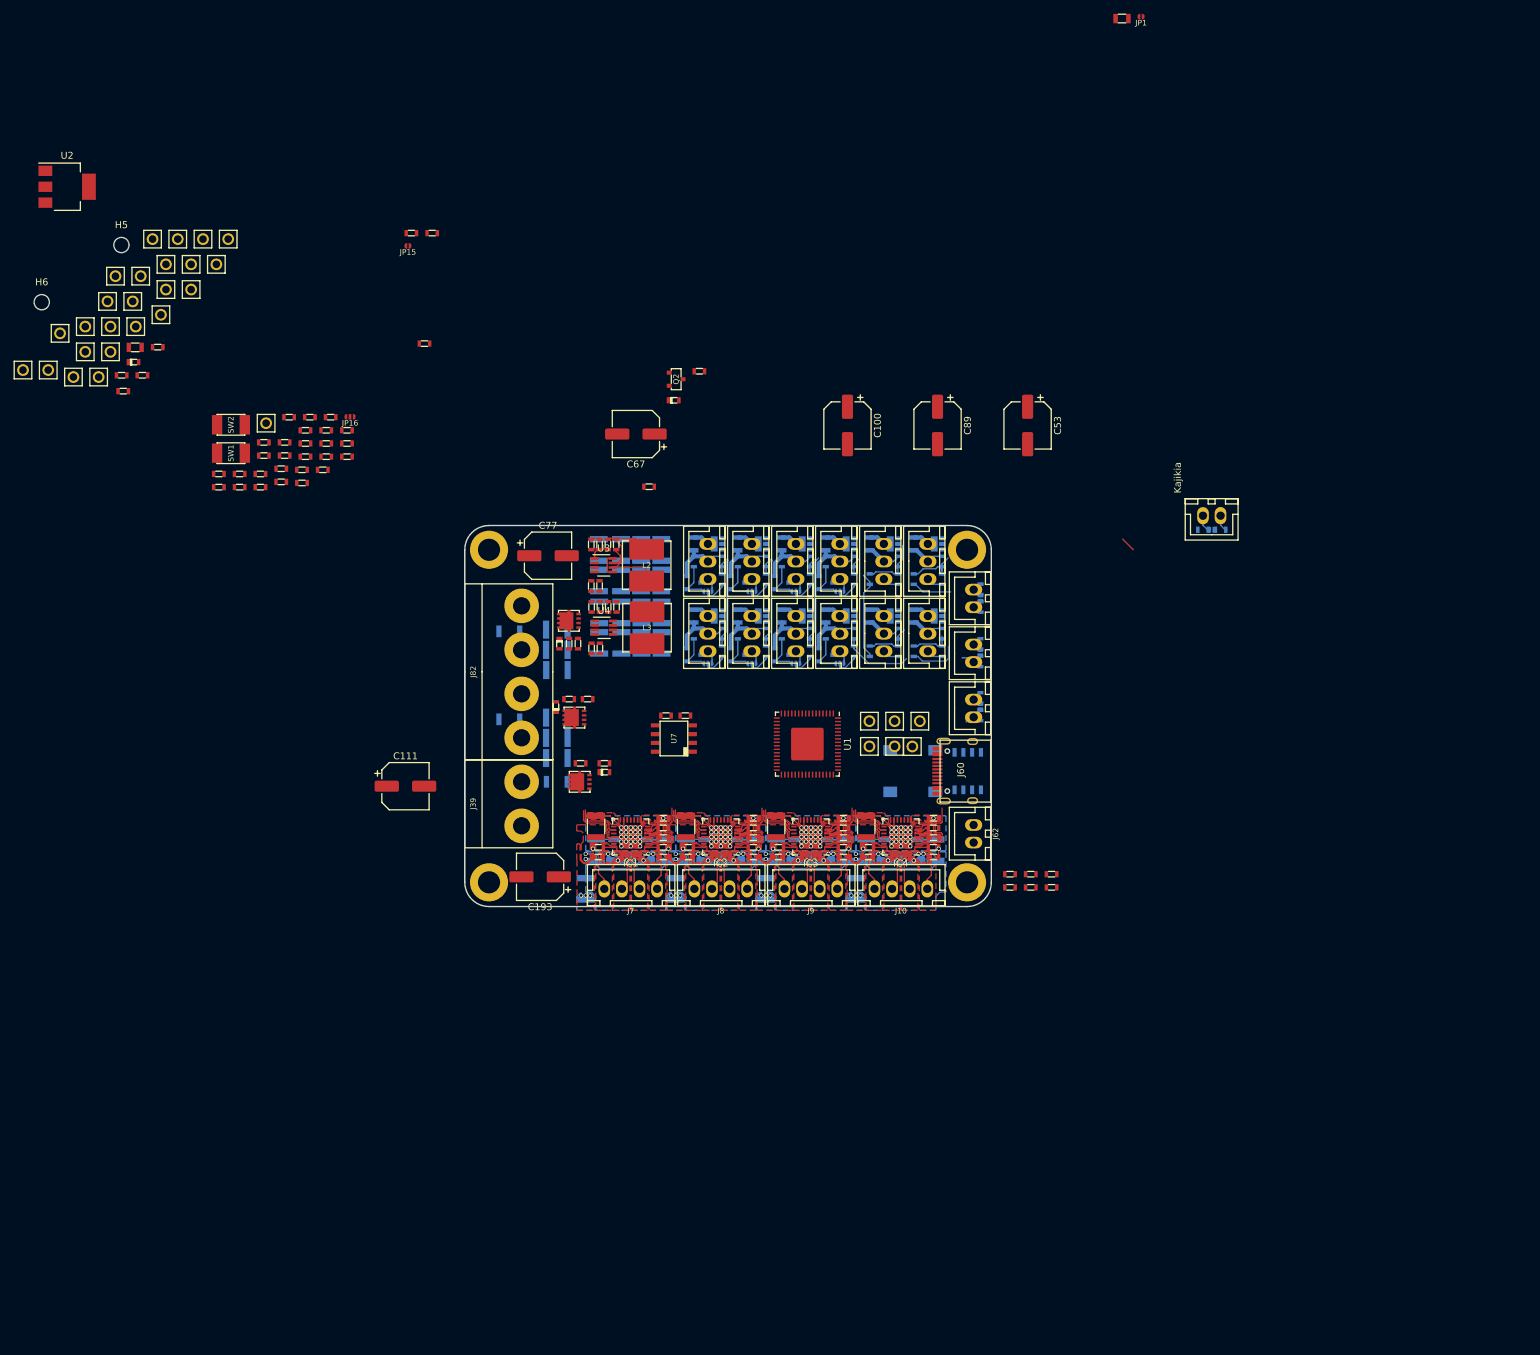
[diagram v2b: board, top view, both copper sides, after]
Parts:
- removed the C73 at (111.9, 125.1)
- removed the C74 at (114.9, 129.2)
- C23, C24, C25, C27, C30, C32, C33, C34, C35, C36, C38, C40, C41, C42, C43, C44, F1, U5: moved to B.Cu
- C3, C5: value 4.7u -> 100n; footprint _Generic:1210_CAP -> _Generic:0603_CAP
- moved C27 85.7 mm to (119.4, 57.9), turned to 90 degrees
- moved C5 74.9 mm to (119.5, 67.7), turned to 90 degrees
- moved C38 73.9 mm to (128.4, 66.9), turned to 90 degrees
- moved C40 70.6 mm to (125.5, 66.9), turned to 90 degrees
- moved C33 68.3 mm to (122.6, 66.9), turned to 90 degrees
- moved C36 67.1 mm to (125.5, 57.9), turned to 90 degrees
- moved C25 66.2 mm to (119.4, 66.9), turned to 90 degrees
- moved C32 64.5 mm to (128.4, 57.9), turned to 90 degrees
- moved C24 63.2 mm to (119.4, 62.5), turned to 270 degrees
- moved C44 63.0 mm to (128.4, 62.5), turned to 270 degrees
- moved C30 61.8 mm to (125.5, 53.5), turned to 270 degrees
- moved D18 59.9 mm to (113.7, 67.1), turned to 270 degrees
- moved C43 59.8 mm to (125.5, 62.5), turned to 270 degrees
- moved R63 59.5 mm to (115.1, 67.1), turned to 90 degrees
- moved C34 59.4 mm to (122.6, 62.5), turned to 270 degrees
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- renumbered C128 to C73, C129 to C74
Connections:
- C30 pad 2: Net-(C30-Pad2) -> GND
- C33 pad 2: Net-(C33-Pad2) -> GND
- C35 pad 2: Net-(C30-Pad2) -> GND
- C38 pad 2: Net-(C33-Pad2) -> GND
- C41 pad 2: Net-(C30-Pad2) -> GND
- C43 pad 2: Net-(C33-Pad2) -> GND
- R63 pad 1: +3V3 -> +12V
- R64 pad 1: +3V3 -> +12V
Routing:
- net Net-(C37-Pad2): track 0.00 -> 11.4 mm
- net +12V: track 0.00 -> 6.24 mm
- net Net-(C39-Pad2): track 0.00 -> 4.19 mm
- net +24V: track 109.8 -> 113.3 mm
- net Net-(C37-Pad1): track 0.00 -> 3.13 mm
- net GND: track 245.3 -> 246.5 mm
